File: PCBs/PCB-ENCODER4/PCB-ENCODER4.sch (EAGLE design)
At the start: 37 parts, among them IC1 MCP23017SS, IC2 74HC14D, SW1 EC12E_SW, SW2 EC12E_SW, SW3 EC12E_SW, SW4 EC12E_SW

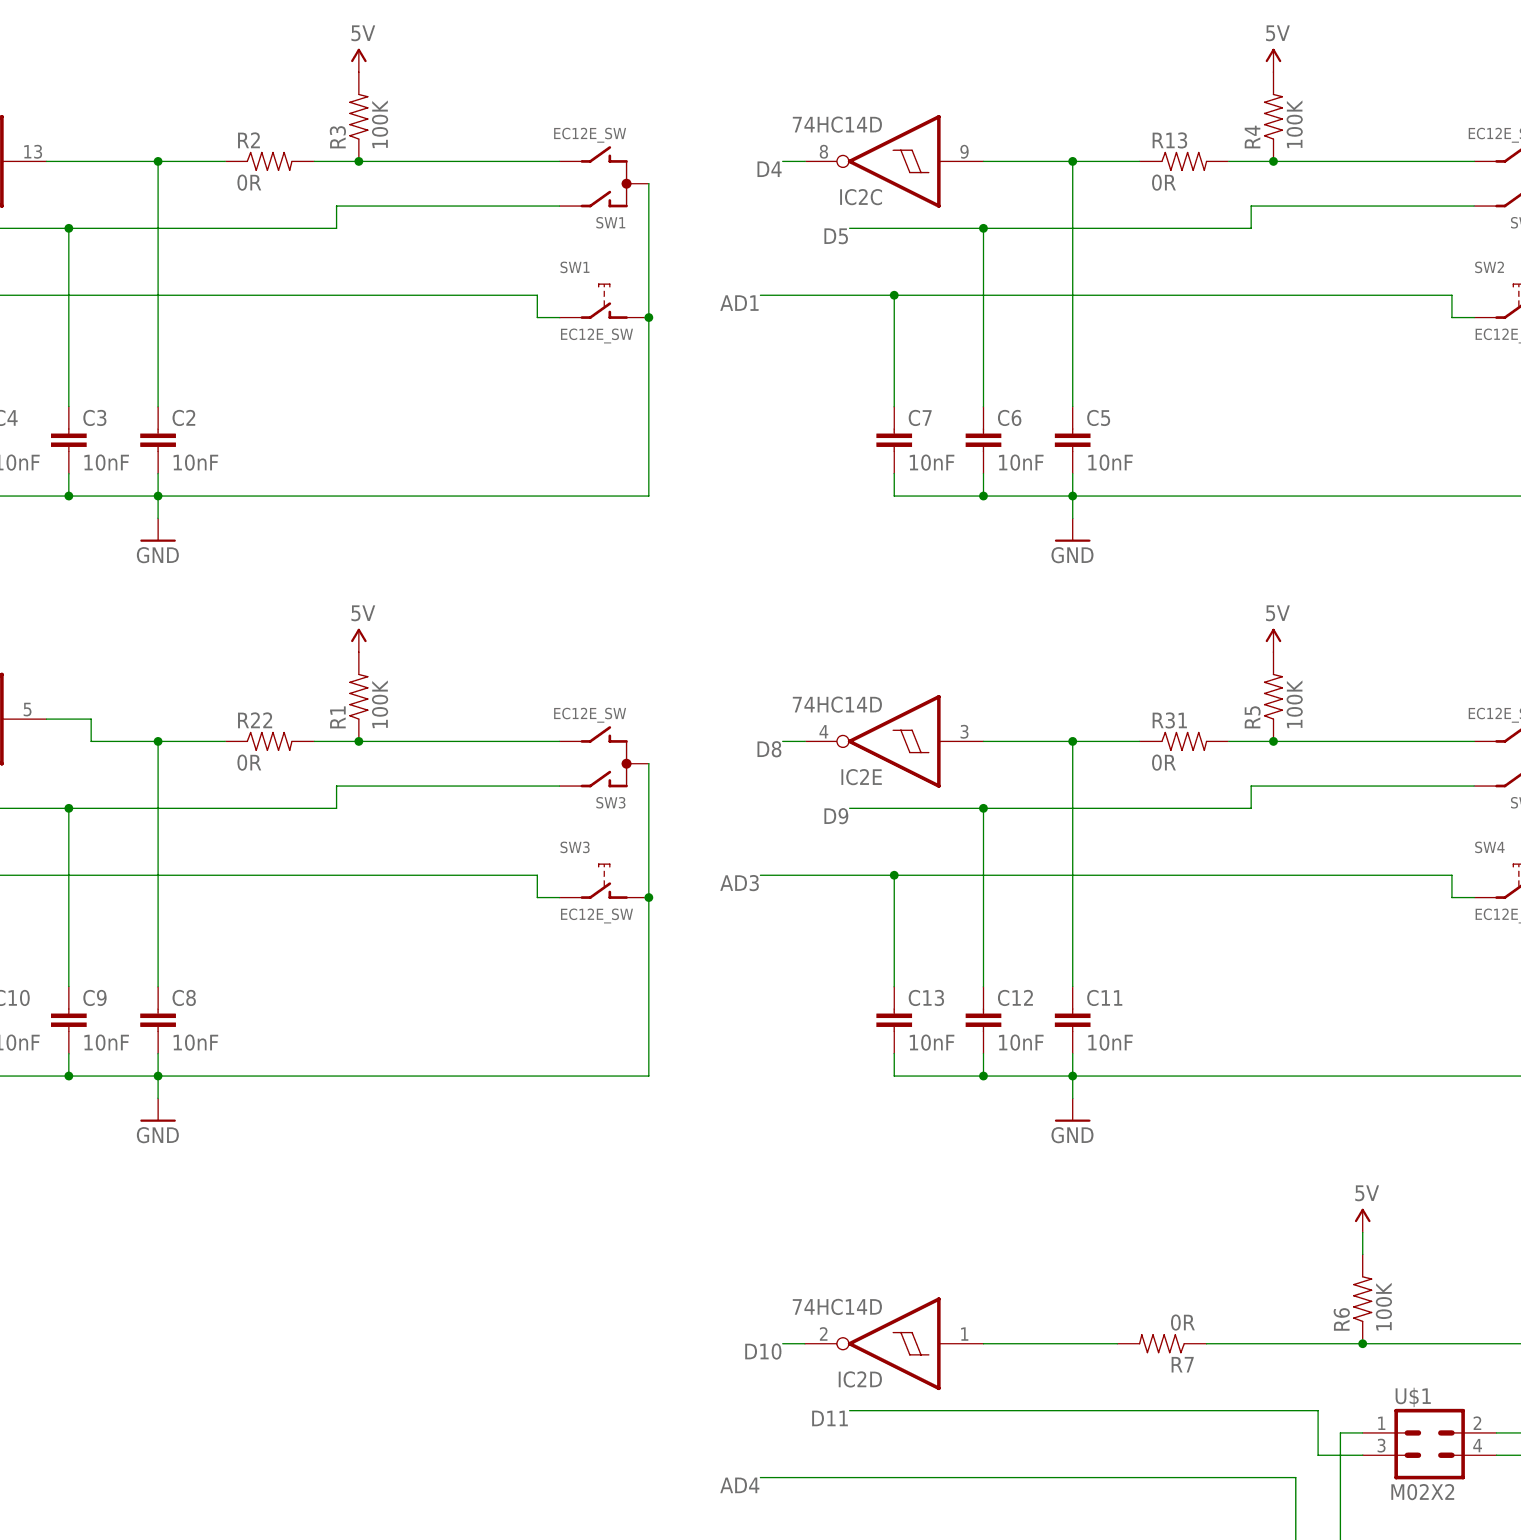
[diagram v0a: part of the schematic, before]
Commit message: asdf
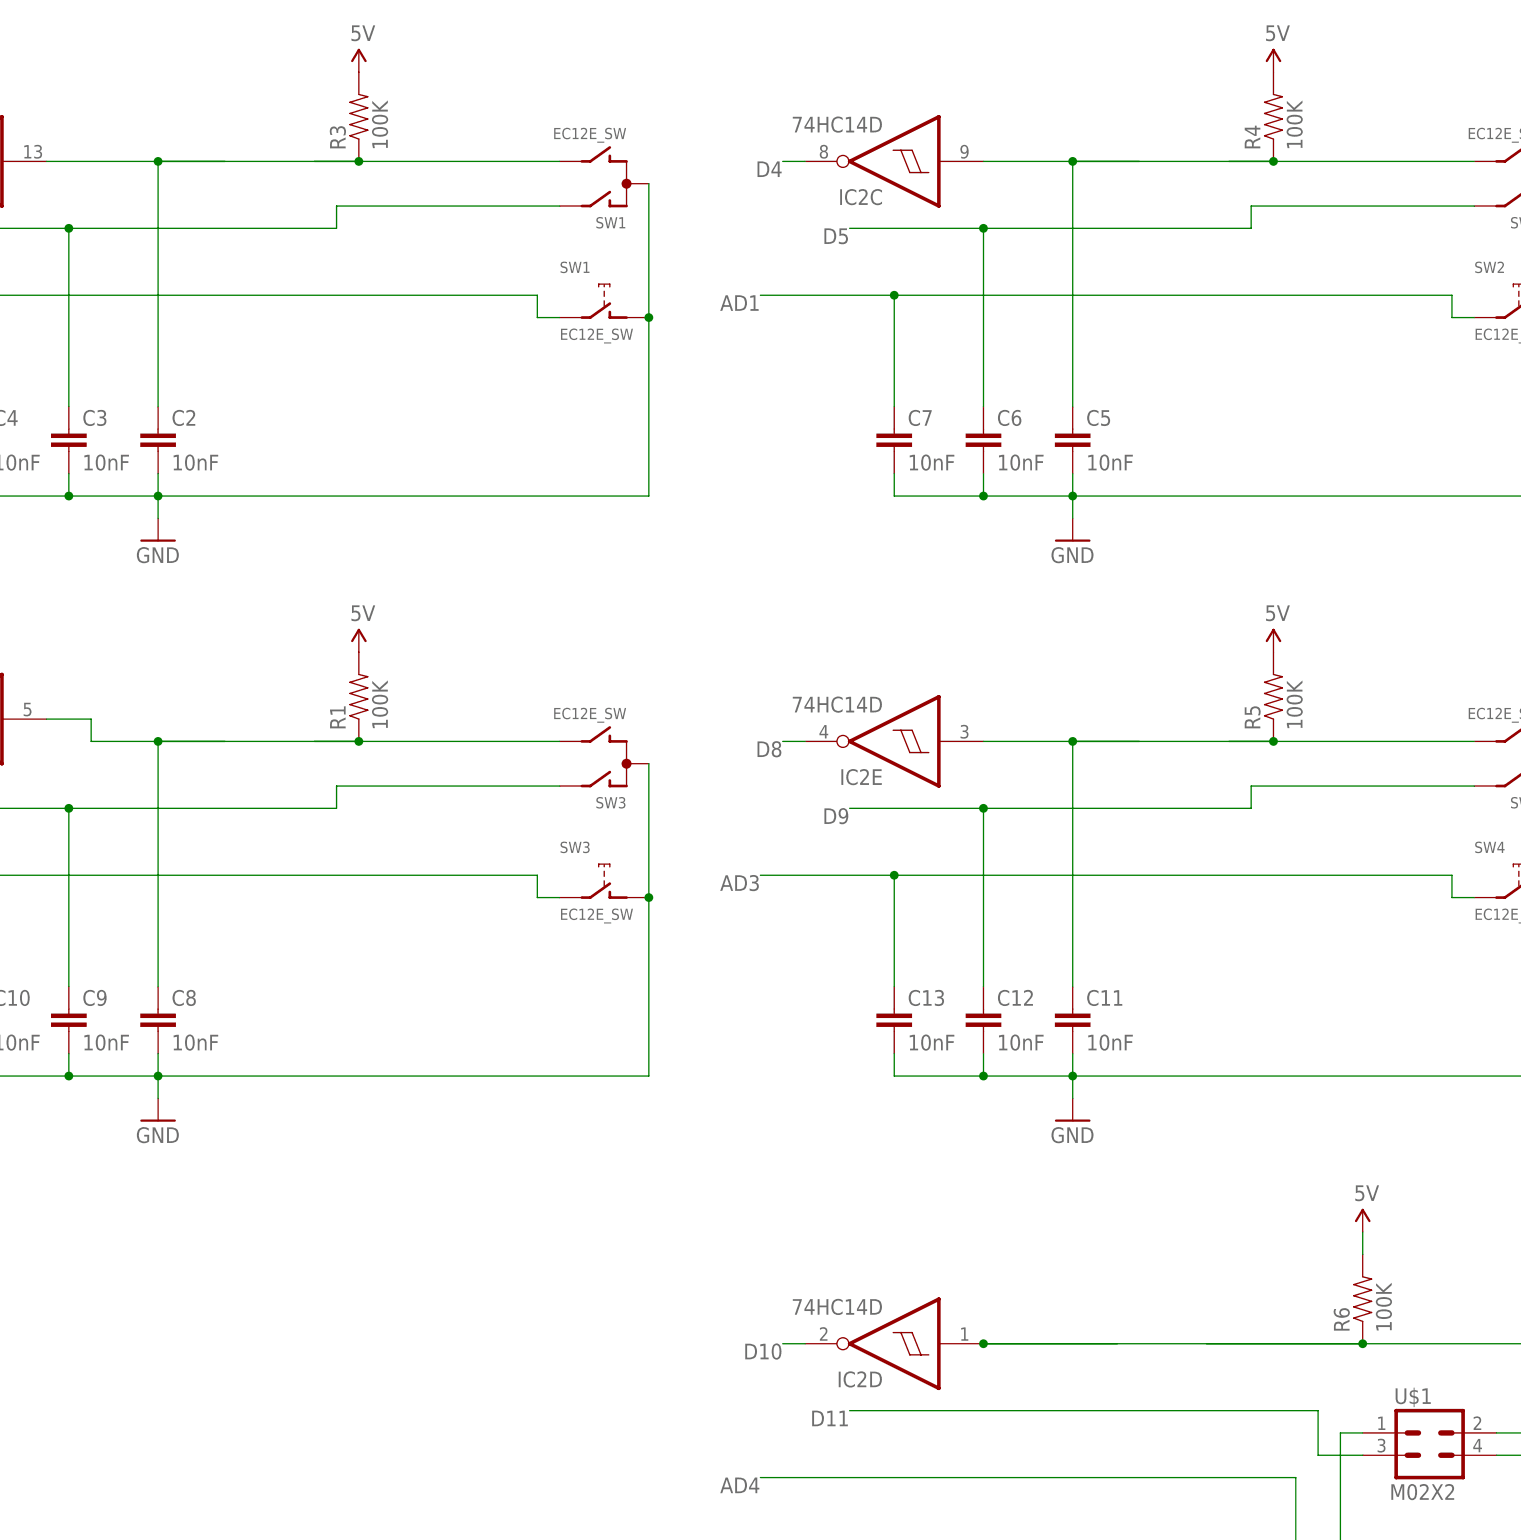
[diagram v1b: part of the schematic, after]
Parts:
- removed R13, R2, R22, R31, R7: 0R, SparkFun:RESISTOR0603-RES
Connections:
- removed net N$1: R2.2, R3.1, SW1G$1.B
- removed net N$12: R31.2, R5.1, SW4G$1.B
- removed net N$127: R6.1, R7.1, U$1.2
- removed net N$6: R13.2, R4.1, SW2G$1.B
- removed net N$9: R1.1, R22.2, SW3G$1.B
- net N$123: now also R1.1, SW3G$1.B; no longer R22.1
- net N$124: now also R3.1, SW1G$1.B; no longer R2.1
- net N$125: now also R4.1, SW2G$1.B; no longer R13.1
- net N$126: now also R5.1, SW4G$1.B; no longer R31.1
- net N$2: now also R6.1, U$1.2; no longer R7.2
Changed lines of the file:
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@@
 <?xml version="1.0" encoding="utf-8"?>
 <!DOCTYPE eagle SYSTEM "eagle.dtd">
-<eagle version="7.1.0">
+<eagle version="7.2.0">
 <drawing>
 <settings>
@@
 <part name="U$2" library="SparkFun" deviceset="5V" device=""/>
 <part name="GND2" library="SparkFun" deviceset="GND" device=""/>
-<part name="R2" library="SparkFun" deviceset="RESISTOR" device="0603-RES" value="0R"/>
 <part name="U$20" library="SKAARHOJ" deviceset="GNDPAD" device="6MM" value="GNDPAD6MM"/>
 <part name="U$21" library="SKAARHOJ" deviceset="GNDPAD" device="6MM" value="GNDPAD6MM"/>
@@
 <part name="C6" library="SparkFun" deviceset="CAP" device="0603-CAP" value="10nF"/>
 <part name="C7" library="SparkFun" deviceset="CAP" device="0603-CAP" value="10nF"/>
-<part name="R13" library="SparkFun" deviceset="RESISTOR" device="0603-RES" value="0R"/>
 <part name="GND4" library="SparkFun" deviceset="GND" device=""/>
 <part name="SW3" library="switch-alps" deviceset="EC12E_SW" device=""/>
@@
 <part name="C9" library="SparkFun" deviceset="CAP" device="0603-CAP" value="10nF"/>
 <part name="C10" library="SparkFun" deviceset="CAP" device="0603-CAP" value="10nF"/>
-<part name="R22" library="SparkFun" deviceset="RESISTOR" device="0603-RES" value="0R"/>
 <part name="GND5" library="SparkFun" deviceset="GND" device=""/>
 <part name="SW4" library="switch-alps" deviceset="EC12E_SW" device=""/>
@@
 <part name="C12" library="SparkFun" deviceset="CAP" device="0603-CAP" value="10nF"/>
 <part name="C13" library="SparkFun" deviceset="CAP" device="0603-CAP" value="10nF"/>
-<part name="R31" library="SparkFun" deviceset="RESISTOR" device="0603-RES" value="0R"/>
 <part name="IC1" library="microchip" deviceset="MCP23017" device="SS">
 <attribute name="MPN" value="MCP23017-E/SS"/>
@@
 <part name="U$5" library="SparkFun" deviceset="5V" device=""/>
 <part name="U$6" library="SparkFun" deviceset="5V" device=""/>
-<part name="R7" library="SparkFun" deviceset="RESISTOR" device="0603-RES" value="0R"/>
 </parts>
 <sheets>
@@
 <instance part="U$2" gate="G$1" x="162.56" y="104.14"/>
 <instance part="GND2" gate="1" x="162.56" y="93.98"/>
-<instance part="R2" gate="G$1" x="-53.34" y="144.78"/>
 <instance part="U$20" gate="G$1" x="147.32" y="73.66"/>
 <instance part="U$21" gate="G$1" x="175.26" y="73.66"/>
@@
 <instance part="C6" gate="G$1" x="27.94" y="111.76"/>
 <instance part="C7" gate="G$1" x="17.78" y="111.76"/>
-<instance part="R13" gate="G$1" x="50.8" y="144.78"/>
 <instance part="GND4" gate="1" x="-66.04" y="35.56"/>
 <instance part="SW3" gate="G$1" x="-12.7" y="76.2" rot="R90"/>
@@
 <instance part="C9" gate="G$1" x="-76.2" y="45.72"/>
 <instance part="C10" gate="G$1" x="-86.36" y="45.72"/>
-<instance part="R22" gate="G$1" x="-53.34" y="78.74"/>
 <instance part="GND5" gate="1" x="38.1" y="35.56"/>
 <instance part="SW4" gate="G$1" x="91.44" y="76.2" rot="R90"/>
@@
 <instance part="C12" gate="G$1" x="27.94" y="45.72"/>
 <instance part="C13" gate="G$1" x="17.78" y="45.72"/>
-<instance part="R31" gate="G$1" x="50.8" y="78.74"/>
 <instance part="IC1" gate="G$1" x="-167.64" y="124.46" rot="R180"/>
 <instance part="U$13" gate="G$1" x="-142.24" y="104.14"/>
@@
 <instance part="U$6" gate="G$1" x="-43.18" y="88.9"/>
 <instance part="IC2" gate="B" x="17.78" y="-27.94" rot="R180"/>
-<instance part="R7" gate="G$1" x="48.26" y="10.16" rot="R180"/>
 </instances>
 <busses>
@@
 </segment>
 </net>
-<net name="N$1" class="0">
-<segment>
-<pinref part="SW1" gate="G$1" pin="B"/>
-<pinref part="R2" gate="G$1" pin="2"/>
-<wire x1="-48.26" y1="144.78" x2="-43.18" y2="144.78" width="0.1524" layer="91"/>
-<pinref part="R3" gate="G$1" pin="1"/>
-<wire x1="-43.18" y1="144.78" x2="-20.32" y2="144.78" width="0.1524" layer="91"/>
-<junction x="-43.18" y="144.78"/>
-</segment>
-</net>
 <net name="I2C_SDA" class="0">
 <segment>
@@
 </segment>
 </net>
-<net name="N$6" class="0">
-<segment>
-<pinref part="SW2" gate="G$1" pin="B"/>
-<pinref part="R13" gate="G$1" pin="2"/>
-<wire x1="55.88" y1="144.78" x2="60.96" y2="144.78" width="0.1524" layer="91"/>
-<pinref part="R4" gate="G$1" pin="1"/>
-<wire x1="60.96" y1="144.78" x2="83.82" y2="144.78" width="0.1524" layer="91"/>
-<junction x="60.96" y="144.78"/>
-</segment>
-</net>
-<net name="N$9" class="0">
-<segment>
-<pinref part="SW3" gate="G$1" pin="B"/>
-<pinref part="R22" gate="G$1" pin="2"/>
-<wire x1="-48.26" y1="78.74" x2="-43.18" y2="78.74" width="0.1524" layer="91"/>
-<pinref part="R1" gate="G$1" pin="1"/>
-<wire x1="-43.18" y1="78.74" x2="-20.32" y2="78.74" width="0.1524" layer="91"/>
-<junction x="-43.18" y="78.74"/>
-</segment>
-</net>
-<net name="N$12" class="0">
-<segment>
-<pinref part="SW4" gate="G$1" pin="B"/>
-<pinref part="R31" gate="G$1" pin="2"/>
-<wire x1="55.88" y1="78.74" x2="60.96" y2="78.74" width="0.1524" layer="91"/>
-<pinref part="R5" gate="G$1" pin="1"/>
-<wire x1="60.96" y1="78.74" x2="83.82" y2="78.74" width="0.1524" layer="91"/>
-<junction x="60.96" y="78.74"/>
-</segment>
-</net>
 <net name="A0" class="0">
 <segment>
@@
 <wire x1="-66.04" y1="50.8" x2="-66.04" y2="78.74" width="0.1524" layer="91"/>
 <wire x1="-66.04" y1="78.74" x2="-58.42" y2="78.74" width="0.1524" layer="91"/>
-<pinref part="R22" gate="G$1" pin="1"/>
 <junction x="-66.04" y="78.74"/>
 <wire x1="-78.74" y1="81.28" x2="-73.66" y2="81.28" width="0.1524" layer="91"/>
@@
 <wire x1="-73.66" y1="78.74" x2="-66.04" y2="78.74" width="0.1524" layer="91"/>
 <pinref part="IC2" gate="F" pin="I"/>
+<pinref part="SW3" gate="G$1" pin="B"/>
+<wire x1="-48.26" y1="78.74" x2="-43.18" y2="78.74" width="0.1524" layer="91"/>
+<pinref part="R1" gate="G$1" pin="1"/>
+<wire x1="-43.18" y1="78.74" x2="-20.32" y2="78.74" width="0.1524" layer="91"/>
+<junction x="-43.18" y="78.74"/>
+<wire x1="-66.04" y1="78.74" x2="-43.18" y2="78.74" width="0.1524" layer="91"/>
 </segment>
 </net>
@@
 <wire x1="-66.04" y1="116.84" x2="-66.04" y2="144.78" width="0.1524" layer="91"/>
 <wire x1="-66.04" y1="144.78" x2="-58.42" y2="144.78" width="0.1524" layer="91"/>
-<pinref part="R2" gate="G$1" pin="1"/>
 <junction x="-66.04" y="144.78"/>
 <pinref part="IC2" gate="A" pin="I"/>
 <wire x1="-78.74" y1="144.78" x2="-66.04" y2="144.78" width="0.1524" layer="91"/>
+<pinref part="SW1" gate="G$1" pin="B"/>
+<wire x1="-48.26" y1="144.78" x2="-43.18" y2="144.78" width="0.1524" layer="91"/>
+<pinref part="R3" gate="G$1" pin="1"/>
+<wire x1="-43.18" y1="144.78" x2="-20.32" y2="144.78" width="0.1524" layer="91"/>
+<junction x="-43.18" y="144.78"/>
+<wire x1="-66.04" y1="144.78" x2="-43.18" y2="144.78" width="0.1524" layer="91"/>
 </segment>
 </net>
@@
 <wire x1="38.1" y1="116.84" x2="38.1" y2="144.78" width="0.1524" layer="91"/>
 <wire x1="38.1" y1="144.78" x2="45.72" y2="144.78" width="0.1524" layer="91"/>
-<pinref part="R13" gate="G$1" pin="1"/>
 <junction x="38.1" y="144.78"/>
 <pinref part="IC2" gate="C" pin="I"/>
 <wire x1="27.94" y1="144.78" x2="38.1" y2="144.78" width="0.1524" layer="91"/>
+<pinref part="SW2" gate="G$1" pin="B"/>
+<wire x1="55.88" y1="144.78" x2="60.96" y2="144.78" width="0.1524" layer="91"/>
+<pinref part="R4" gate="G$1" pin="1"/>
+<wire x1="60.96" y1="144.78" x2="83.82" y2="144.78" width="0.1524" layer="91"/>
+<junction x="60.96" y="144.78"/>
+<wire x1="38.1" y1="144.78" x2="60.96" y2="144.78" width="0.1524" layer="91"/>
 </segment>
 </net>
@@
 <wire x1="38.1" y1="50.8" x2="38.1" y2="78.74" width="0.1524" layer="91"/>
 <wire x1="38.1" y1="78.74" x2="45.72" y2="78.74" width="0.1524" layer="91"/>
-<pinref part="R31" gate="G$1" pin="1"/>
 <junction x="38.1" y="78.74"/>
 <pinref part="IC2" gate="E" pin="I"/>
 <wire x1="38.1" y1="78.74" x2="27.94" y2="78.74" width="0.1524" layer="91"/>
-</segment>
-</net>
-<net name="N$127" class="0">
-<segment>
+<pinref part="SW4" gate="G$1" pin="B"/>
+<wire x1="55.88" y1="78.74" x2="60.96" y2="78.74" width="0.1524" layer="91"/>
+<pinref part="R5" gate="G$1" pin="1"/>
+<wire x1="60.96" y1="78.74" x2="83.82" y2="78.74" width="0.1524" layer="91"/>
+<junction x="60.96" y="78.74"/>
+<wire x1="38.1" y1="78.74" x2="60.96" y2="78.74" width="0.1524" layer="91"/>
+</segment>
+</net>
+<net name="N$2" class="0">
+<segment>
+<pinref part="IC2" gate="D" pin="I"/>
+<wire x1="43.18" y1="10.16" x2="27.94" y2="10.16" width="0.1524" layer="91"/>
 <pinref part="R6" gate="G$1" pin="1"/>
 <pinref part="U$1" gate="G$1" pin="2"/>
@@
 <wire x1="93.98" y1="0" x2="93.98" y2="10.16" width="0.1524" layer="91"/>
 <wire x1="93.98" y1="10.16" x2="71.12" y2="10.16" width="0.1524" layer="91"/>
-<pinref part="R7" gate="G$1" pin="1"/>
 <wire x1="53.34" y1="10.16" x2="71.12" y2="10.16" width="0.1524" layer="91"/>
 <junction x="71.12" y="10.16"/>
-</segment>
-</net>
-<net name="N$2" class="0">
-<segment>
-<pinref part="R7" gate="G$1" pin="2"/>
-<pinref part="IC2" gate="D" pin="I"/>
-<wire x1="43.18" y1="10.16" x2="27.94" y2="10.16" width="0.1524" layer="91"/>
-</segment>
-</net>
+<wire x1="27.94" y1="10.16" x2="71.12" y2="10.16" width="0.1524" layer="91"/>
+<junction x="27.94" y="10.16"/>
+</segment>
+</net>
